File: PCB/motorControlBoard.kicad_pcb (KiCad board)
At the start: 2 copper layers, 62.5 x 79.5 mm, 12 parts, among them J1 Barrel_Jack, J2 B5B-XH-ALFSN, J3 B5B-XH-ALFSN, J4 B5B-XH-ALFSN, U1 ULN2003A, U2 ULN2003A, U3 ULN2003A

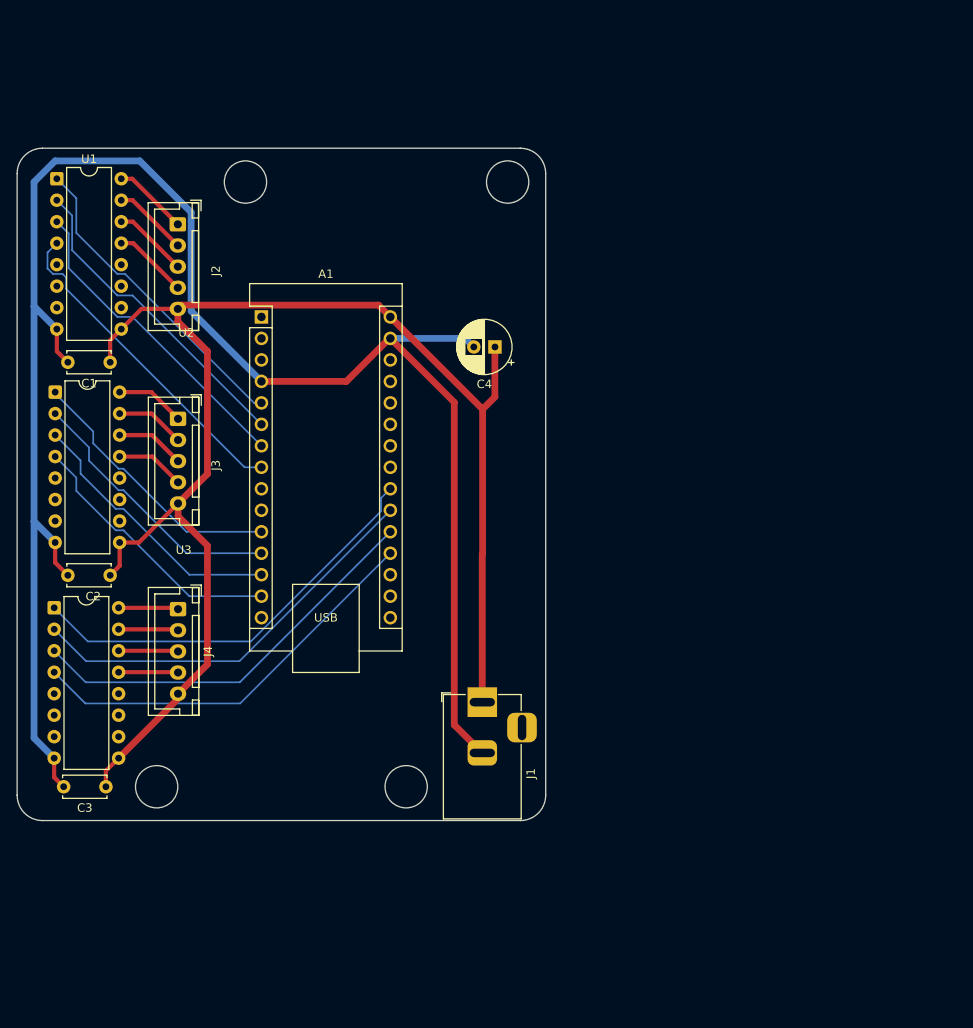
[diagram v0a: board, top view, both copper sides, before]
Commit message: final (i think)
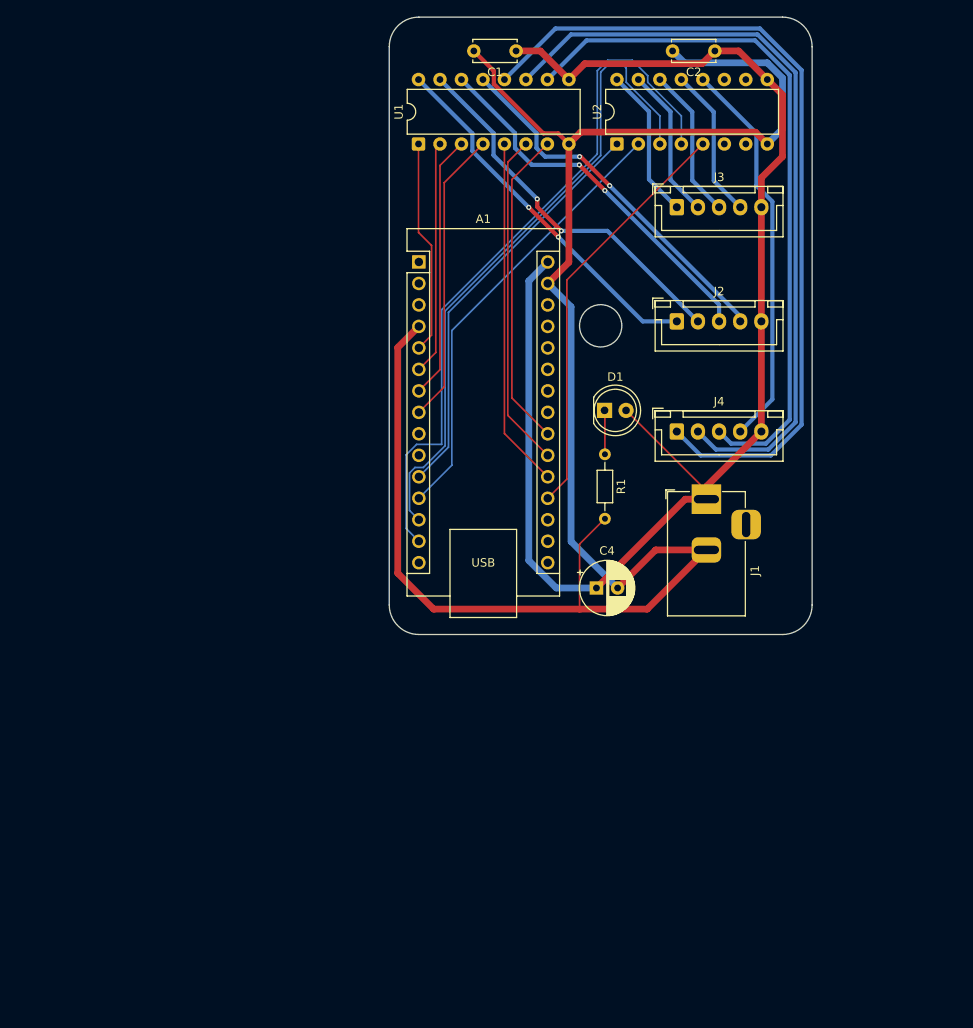
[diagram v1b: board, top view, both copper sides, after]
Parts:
- removed C3: 100nF, Capacitor_THT:C_Disc_D5.0mm_W2.5mm_P5.00mm
- removed U3: ULN2003A, Package_DIP:DIP-16_W7.62mm
- added D1: LED, LED_THT:LED_D5.0mm, F.Cu at (133.5, 66.0)
- added R1: 220 Ohm, Resistor_THT:R_Axial_DIN0204_L3.6mm_D1.6mm_P7.62mm_Horizontal, F.Cu at (133.5, 71.2)
- moved C2 94.6 mm to (146.5, 23.5)
- moved U2 72.6 mm to (134.9, 34.5), turned to 90 degrees
- moved J3 64.1 mm to (142.0, 42.0), turned to 0 degrees
- moved J4 62.6 mm to (142.0, 68.5), turned to 0 degrees
- moved C1 60.5 mm to (123.0, 23.5)
- moved J2 60.1 mm to (142.0, 55.5), turned to 0 degrees
- moved U1 43.0 mm to (111.5, 34.5), turned to 90 degrees
- moved J1 35.8 mm to (145.5, 76.5)
- moved C4 30.9 mm to (132.5, 87.0), turned to 0 degrees
- moved A1 19.7 mm to (111.5, 48.5)
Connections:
- J4 pad 1: Net-(U3-O1) -> Net-(U1-O5)
- J4 pad 2: Net-(U3-O2) -> Net-(U1-O6)
- J4 pad 3: Net-(U3-O3) -> Net-(U1-O7)
- J4 pad 4: Net-(U3-O4) -> Net-(U2-O5)
- U1 pad 10: unconnected-(U1-O7-Pad10) -> Net-(U1-O7)
- U1 pad 11: unconnected-(U1-O6-Pad11) -> Net-(U1-O6)
- U1 pad 12: unconnected-(U1-O5-Pad12) -> Net-(U1-O5)
- U1 pad 5: unconnected-(U1-I5-Pad5) -> Net-(A1-A1)
- U1 pad 6: unconnected-(U1-I6-Pad6) -> Net-(A1-A2)
- U1 pad 7: unconnected-(U1-I7-Pad7) -> Net-(A1-A3)
- U2 pad 12: unconnected-(U2-O5-Pad12) -> Net-(U2-O5)
- U2 pad 5: unconnected-(U2-I5-Pad5) -> Net-(A1-A0)
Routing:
- net Net-(U1-O5): track 0.00 -> 99.0 mm
- net Net-(U1-O6): track 0.00 -> 91.1 mm
- net Net-(U1-O7): track 0.00 -> 83.1 mm
- net Net-(A1-D11): track 32.1 -> 84.3 mm
- net Net-(U2-O5): track 0.00 -> 46.6 mm
- net Net-(A1-D10): track 32.1 -> 77.6 mm
- net Net-(U1-O3): track 8.88 -> 44.5 mm, vias 0 -> 2
- net Net-(U1-O2): track 8.90 -> 44.4 mm, vias 0 -> 2
- net Net-(U1-O4): track 8.87 -> 43.7 mm, vias 0 -> 2
- net Net-(U1-O1): track 8.92 -> 43.6 mm, vias 0 -> 2
- net Net-(A1-D9): track 32.1 -> 52.6 mm
- net Net-(A1-D8): track 32.1 -> 49.1 mm
- net Net-(A1-D2): track 37.6 -> 25.4 mm
- net Net-(A1-A3): track 49.8 -> 37.8 mm
- net Net-(A1-VIN): track 175.8 -> 165.4 mm
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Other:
- board size 62.5 x 79.5 mm -> 50 x 73 mm

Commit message: final final final
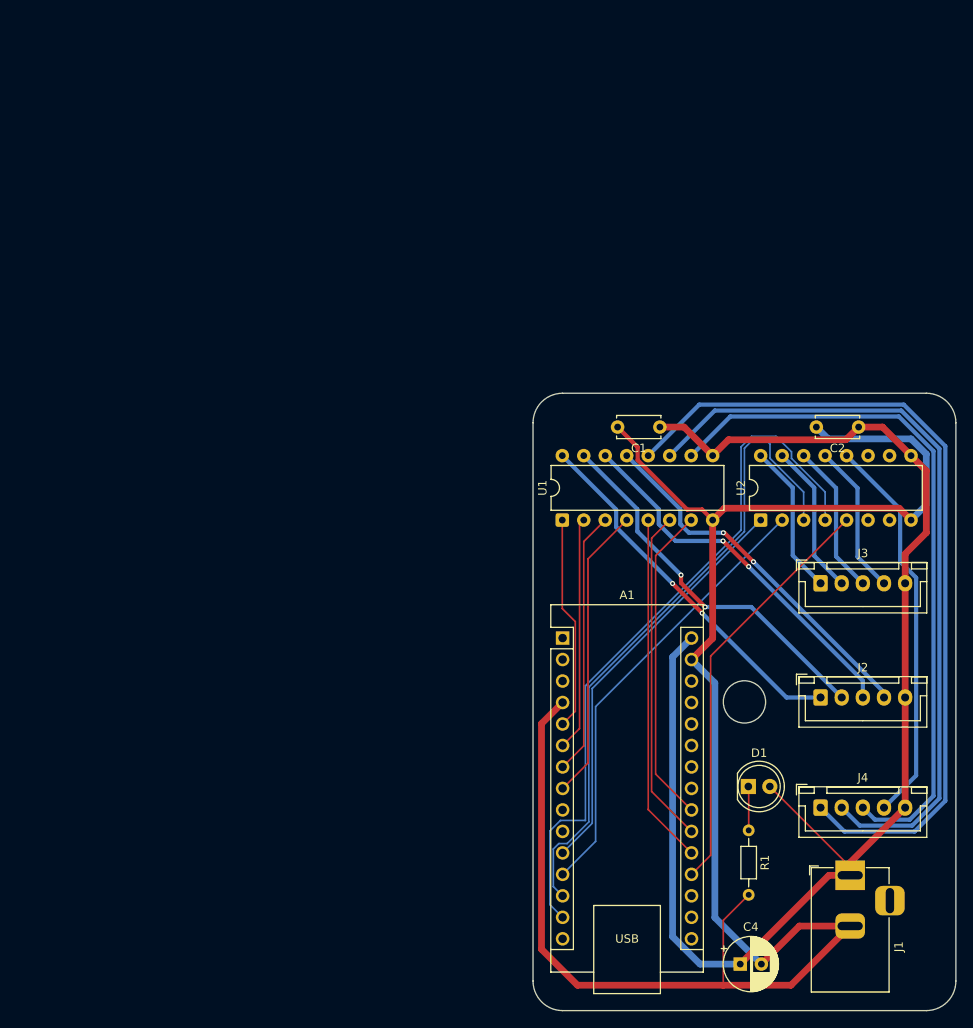
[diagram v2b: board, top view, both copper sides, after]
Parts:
- moved A1 47.6 mm to (128.5, 92.9)
- moved C1 47.6 mm to (140.0, 68.0)
- moved C2 47.6 mm to (163.5, 68.0)
- moved C4 47.6 mm to (149.5, 131.5)
- moved D1 47.6 mm to (150.5, 110.5)
- moved J1 47.6 mm to (162.5, 121.0)
- moved J4 47.6 mm to (159.0, 113.0)
- moved R1 47.6 mm to (150.5, 115.7)
- moved U1 47.6 mm to (128.5, 79.0)
- moved U2 47.6 mm to (151.9, 79.0)
- moved J2 47.6 mm to (159.0, 99.9)
- moved J3 47.6 mm to (159.0, 86.4)
